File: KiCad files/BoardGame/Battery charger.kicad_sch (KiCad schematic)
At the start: 15 parts, among them J301 Conn_01x01, J302 Conn_01x01, U301 MCP73871-2CC

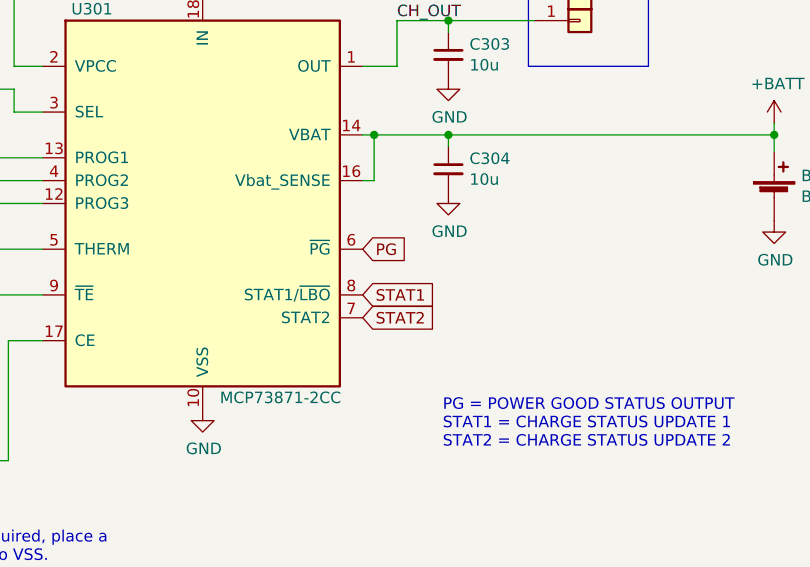
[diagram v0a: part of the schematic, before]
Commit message: Schematic update
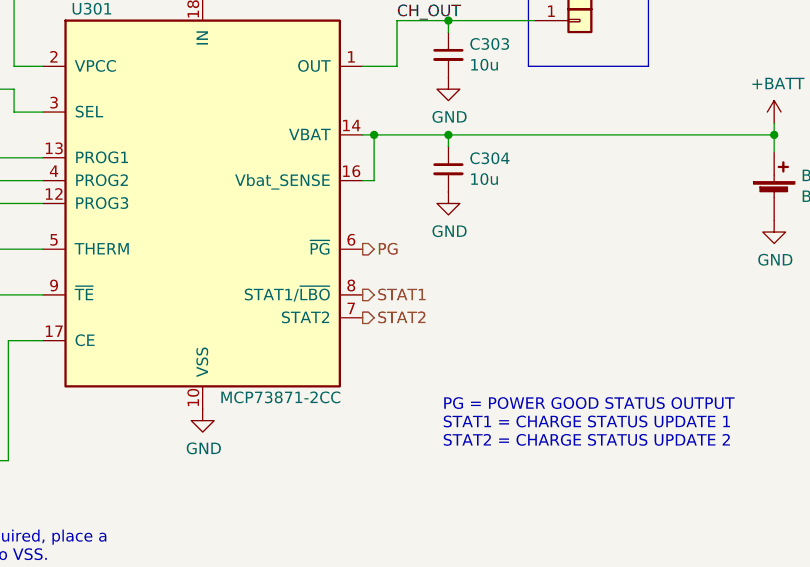
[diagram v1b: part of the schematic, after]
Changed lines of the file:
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@@
     (effects (font (size 1.27 1.27)) (justify left bottom))
   )
-  (global_label "PG" (shape input) (at 156.21 86.995 0) (fields_autoplaced)
+  (hierarchical_label "STAT2" (shape output) (at 156.21 94.615 0)
     (effects (font (size 1.27 1.27)) (justify left))
-    (property "Intersheet References" "${INTERSHEET_REFS}" (id 0) (at 161.1631 86.9156 0)
-      (effects (font (size 1.27 1.27)) (justify left) hide)
-    )
   )
-  (global_label "STAT1" (shape input) (at 156.21 92.075 0) (fields_autoplaced)
+  (hierarchical_label "PG" (shape output) (at 156.21 86.995 0)
     (effects (font (size 1.27 1.27)) (justify left))
-    (property "Intersheet References" "${INTERSHEET_REFS}" (id 0) (at 164.066 91.9956 0)
-      (effects (font (size 1.27 1.27)) (justify left) hide)
-    )
   )
-  (global_label "STAT2" (shape input) (at 156.21 94.615 0) (fields_autoplaced)
+  (hierarchical_label "STAT1" (shape output) (at 156.21 92.075 0)
     (effects (font (size 1.27 1.27)) (justify left))
-    (property "Intersheet References" "${INTERSHEET_REFS}" (id 0) (at 164.066 94.5356 0)
-      (effects (font (size 1.27 1.27)) (justify left) hide)
-    )
   )
   (symbol (lib_id "power:GND") (at 76.835 62.865 0) (unit 1)
